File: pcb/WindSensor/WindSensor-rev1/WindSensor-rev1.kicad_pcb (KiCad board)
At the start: 2 copper layers, 20 x 20 mm, 18 parts, among them J1 Conn_I2C_Molex_705450003, U1 SDP320x21, U2 SDP320x22, U3 SDP320x23, U4 LP5814DRLR

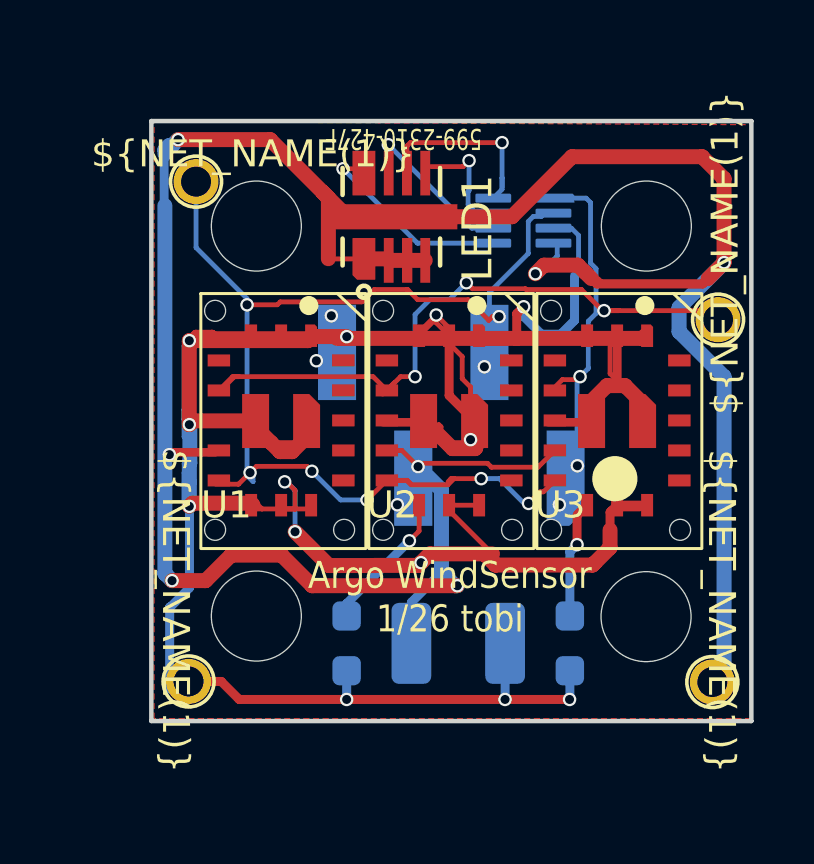
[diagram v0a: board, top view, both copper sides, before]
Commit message: wind sensor rev 1 pcb
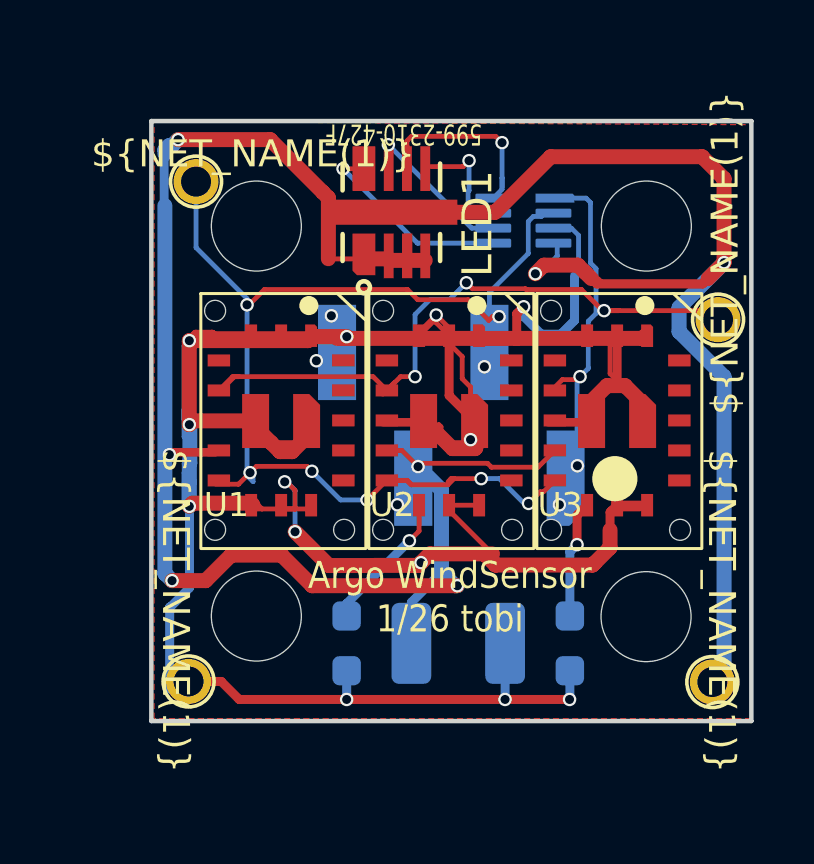
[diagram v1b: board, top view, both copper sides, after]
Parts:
- moved LED1 0.15 mm to (92.8, 79.2)
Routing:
- net VDD: track 109.5 -> 96.3 mm
- net /R: track 6.41 -> 7.44 mm
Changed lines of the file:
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@@
 		(grid_origin 84.81 96.17)
 		(pcbplotparams
-			(layerselection 0x00000000_00000000_5555555f_ffffffff)
+			(layerselection 0x00000000_00000000_55555555_5755f5ff)
 			(plot_on_all_layers_selection 0x00000000_00000000_00000000_00000000)
 			(disableapertmacros no)
 			(usegerberextensions yes)
-			(usegerberattributes no)
-			(usegerberadvancedattributes no)
+			(usegerberattributes yes)
+			(usegerberadvancedattributes yes)
 			(creategerberjobfile no)
 			(dashed_line_dash_ratio 12.000000)
@@
 			(effects
 				(font
-					(size 0.9 0.9)
+					(size 0.8 0.8)
 					(thickness 0.09)
 				)
@@
 			(effects
 				(font
-					(size 0.9 0.9)
+					(size 0.8 0.8)
 					(thickness 0.09)
 				)
@@
 			(effects
 				(font
-					(size 0.9 0.9)
+					(size 0.8 0.8)
 					(thickness 0.09)
 				)
@@
 	(footprint "WindSensor:599-2310_DIA_hand_solder"
 		(layer "F.Cu")
-		(at 92.81 79.37 90)
+		(at 92.81 79.22 90)
 		(tags "599-2310-427F ")
 		(property "Reference" "LED1"
@@
 	)
 	(segment
-		(start 103.169 77.369)
-		(end 98.831 77.369)
+		(start 98.121 77.369)
+		(end 96.27 79.22)
 		(width 0.5)
 		(layer "F.Cu")
@@
 	)
 	(segment
-		(start 91.342268 79.37)
-		(end 90.526134 78.553866)
-		(width 0.5)
+		(start 90.71 80.77)
+		(end 90.7144 80.7744)
+		(width 0.16)
 		(layer "F.Cu")
 		(net 1)
 	)
 	(segment
-		(start 90.71 80.77)
-		(end 90.7144 80.7744)
-		(width 0.16)
+		(start 103.9 78.1)
+		(end 103.169 77.369)
+		(width 0.5)
 		(layer "F.Cu")
 		(net 1)
@@
 	)
 	(segment
+		(start 96.27 79.22)
+		(end 92.81 79.22)
+		(width 0.5)
+		(layer "F.Cu")
+		(net 1)
+	)
+	(segment
 		(start 92.6711 80.7744)
 		(end 92.7211 80.8244)
@@
 	)
 	(segment
+		(start 103.9 80.9)
+		(end 103.9 78.1)
+		(width 0.5)
+		(layer "F.Cu")
+		(net 1)
+	)
+	(segment
 		(start 92.7211 80.8244)
 		(end 93.9403 80.8244)
@@
 	)
 	(segment
+		(start 103.169 77.369)
+		(end 98.121 77.369)
+		(width 0.5)
+		(layer "F.Cu")
+		(net 1)
+	)
+	(segment
 		(start 96.016664 87.589)
 		(end 96.146664 87.719)
@@
 	)
 	(segment
-		(start 103.9 78.1)
-		(end 103.169 77.369)
-		(width 0.5)
-		(layer "F.Cu")
-		(net 1)
-	)
-	(segment
 		(start 90.526134 78.553866)
 		(end 90.71 78.737732)
@@
 	)
 	(segment
-		(start 98.831 77.369)
-		(end 96.83 79.37)
-		(width 0.5)
-		(layer "F.Cu")
-		(net 1)
-	)
-	(segment
 		(start 85.8 76.7)
 		(end 85.6 76.9)
@@
 	)
 	(segment
-		(start 96.83 79.37)
-		(end 91.342268 79.37)
-		(width 0.5)
-		(layer "F.Cu")
-		(net 1)
-	)
-	(segment
 		(start 97.896256 80.983744)
 		(end 97.61 81.27)
@@
 	)
 	(segment
-		(start 103.9 80.9)
-		(end 103.9 78.1)
-		(width 0.5)
-		(layer "F.Cu")
-		(net 1)
-	)
-	(segment
 		(start 103.259 81.541)
 		(end 103.369 81.431)
@@
 	)
 	(segment
-		(start 103.9 90.7)
-		(end 103.9 91.3)
-		(width 0.16)
-		(layer "B.Cu")
-		(net 1)
-	)
-	(segment
 		(start 85.4 87.31)
 		(end 85.41 87.3)
@@
 	)
 	(segment
-		(start 103.9 91.3)
-		(end 103.9 84.7)
-		(width 0.16)
-		(layer "B.Cu")
-		(net 1)
-	)
-	(segment
-		(start 103.9 91.3)
-		(end 103.9 94.6)
-		(width 0.16)
-		(layer "B.Cu")
-		(net 1)
-	)
-	(segment
 		(start 103.9 94.6)
 		(end 103.9 84.7)
@@
 	)
 	(segment
-		(start 93.334174 88.16)
-		(end 93.478174 88.304)
+		(start 96.057913 82.822087)
+		(end 96.18 82.7)
 		(width 0.16)
 		(layer "F.Cu")
@@
 	)
 	(segment
-		(start 95.369993 82.134167)
-		(end 96.057913 82.822087)
+		(start 93.334174 88.16)
+		(end 93.478174 88.304)
 		(width 0.16)
 		(layer "F.Cu")
@@
 	)
 	(segment
-		(start 88 82.305)
-		(end 89.01 82.305)
-		(width 0.16)
-		(layer "F.Cu")
-		(net 4)
-	)
-	(segment
 		(start 95.805 88.1)
 		(end 94.9 88.1)
@@
 	)
 	(segment
-		(start 92.7 88.155)
-		(end 93.329174 88.155)
+		(start 88 82.305)
+		(end 88.069 82.305)
 		(width 0.16)
 		(layer "F.Cu")
@@
 	)
 	(segment
-		(start 93.346706 81.794)
-		(end 93.366353 81.813647)
+		(start 92.7 88.155)
+		(end 93.329174 88.155)
 		(width 0.16)
 		(layer "F.Cu")
@@
 	)
 	(segment
-		(start 89.107 82.208)
-		(end 91.826494 82.208)
+		(start 88.069 82.305)
+		(end 88.58 81.794)
 		(width 0.16)
 		(layer "F.Cu")
@@
 	)
 	(segment
-		(start 93.346705 81.794)
-		(end 93.366353 81.813647)
+		(start 86.95 88.285)
+		(end 87.715 88.285)
 		(width 0.16)
 		(layer "F.Cu")
@@
 	)
 	(segment
-		(start 86.95 88.285)
-		(end 87.715 88.285)
+		(start 95.369993 82.134167)
+		(end 96.057913 82.822087)
 		(width 0.16)
 		(layer "F.Cu")
@@
 	)
 	(segment
-		(start 96.057913 82.822087)
-		(end 96.18 82.7)
-		(width 0.16)
-		(layer "F.Cu")
-		(net 4)
-	)
-	(segment
 		(start 87.715 88.285)
 		(end 88.1 87.9)
@@
 	)
 	(segment
-		(start 92.240494 81.794)
-		(end 93.346706 81.794)
-		(width 0.16)
-		(layer "F.Cu")
-		(net 4)
-	)
-	(segment
-		(start 91.826494 82.208)
-		(end 92.240494 81.794)
+		(start 93.329174 88.155)
+		(end 93.478174 88.304)
 		(width 0.16)
 		(layer "F.Cu")
@@
 	)
 	(segment
-		(start 93.329174 88.155)
-		(end 93.478174 88.304)
+		(start 88.58 81.794)
+		(end 93.346705 81.794)
 		(width 0.16)
 		(layer "F.Cu")
@@
 	)
 	(segment
-		(start 93.366353 81.813647)
+		(start 93.346705 81.794)
 		(end 93.686872 82.134167)
 		(width 0.16)
@@
 	)
 	(segment
-		(start 89.01 82.305)
-		(end 89.107 82.208)
-		(width 0.16)
-		(layer "F.Cu")
-		(net 4)
-	)
-	(segment
 		(start 97.88 88.54)
 		(end 98.26 88.16)
@@
 	)
 	(segment
-		(start 93.3307 77.01)
-		(end 93.4407 76.9)
+		(start 93.3307 76.8393)
+		(end 93.48 76.69)
+		(width 0.16)
+		(layer "F.Cu")
+		(net 6)
+	)
+	(segment
+		(start 93.48 76.69)
+		(end 96.29 76.69)
 		(width 0.16)
 		(layer "F.Cu")
@@
 	)
 	(segment
-		(start 93.4407 76.9)
+		(start 96.29 76.69)
 		(end 96.5 76.9)
 		(width 0.16)
 		(layer "F.Cu")
+		(net 6)
+	)
+	(segment
+		(start 93.3307 77.7656)
+		(end 93.3307 76.8393)
+		(width 0.16)
+		(layer "F.Cu")
